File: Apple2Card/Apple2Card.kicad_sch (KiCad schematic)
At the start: 57 parts, among them J2 Conn_01x25, J3 Conn_01x25, U2 74HCT32, U3 74HCT00, U4 82C55A, U9 28C256

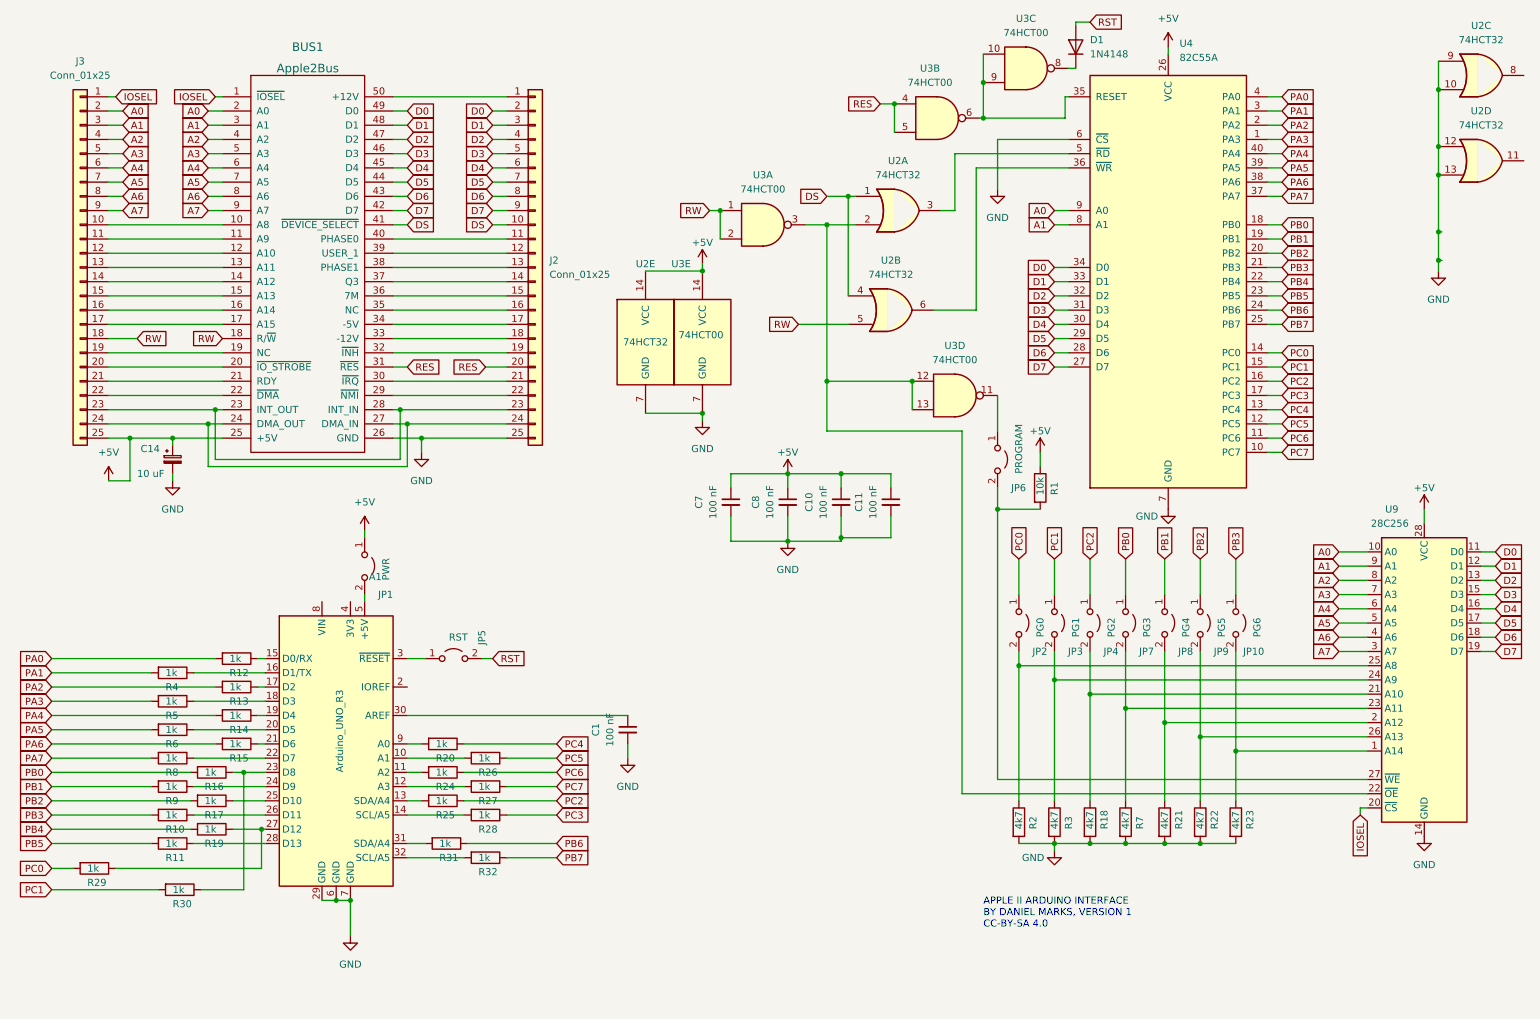
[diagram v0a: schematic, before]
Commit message: JLCPCB Order 2022-06-15
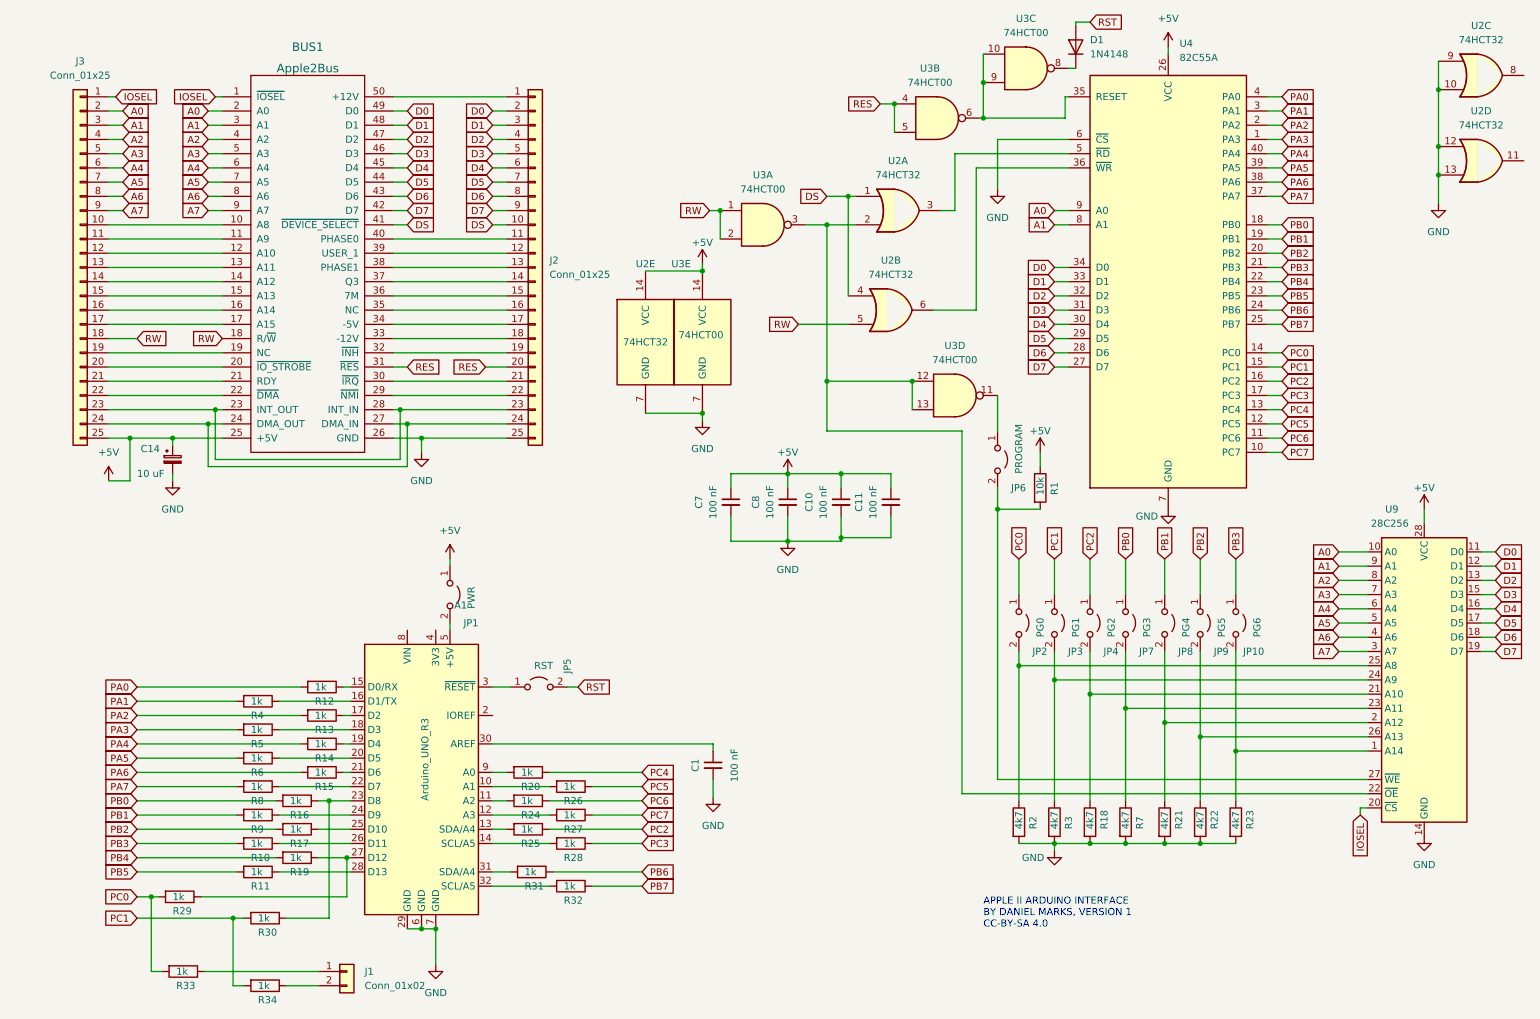
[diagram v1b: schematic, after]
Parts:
- added J1: Conn_01x02, Connector_PinSocket_2.54mm:PinSocket_1x02_P2.54mm_Vertical, symbol Connector_Generic:Conn_01x02
- added R33, R34: 1k, Resistor_THT:R_Axial_DIN0207_L6.3mm_D2.5mm_P7.62mm_Horizontal, symbol Device:R
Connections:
- net PC0: now also R33.2
- net PC1: now also R34.2
- new net: J1.1 (Pin_1), R33.1
- new net: J1.2 (Pin_2), R34.1
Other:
- moved on the sheet: A1, C1, JP1, JP5, R10, R11, R12, R13, R14, R15, R16, R17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
